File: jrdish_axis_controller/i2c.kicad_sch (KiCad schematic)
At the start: 18 parts, among them CN7 SM04B-SRSS-TB (LF)(SN), CN8 SM04B-SRSS-TB (LF)(SN), U5 LTC4311ISC6#TRPBF, U6 LM75BIMX-5/NOPB, U7 W25Q32JVSSIQ_C179173

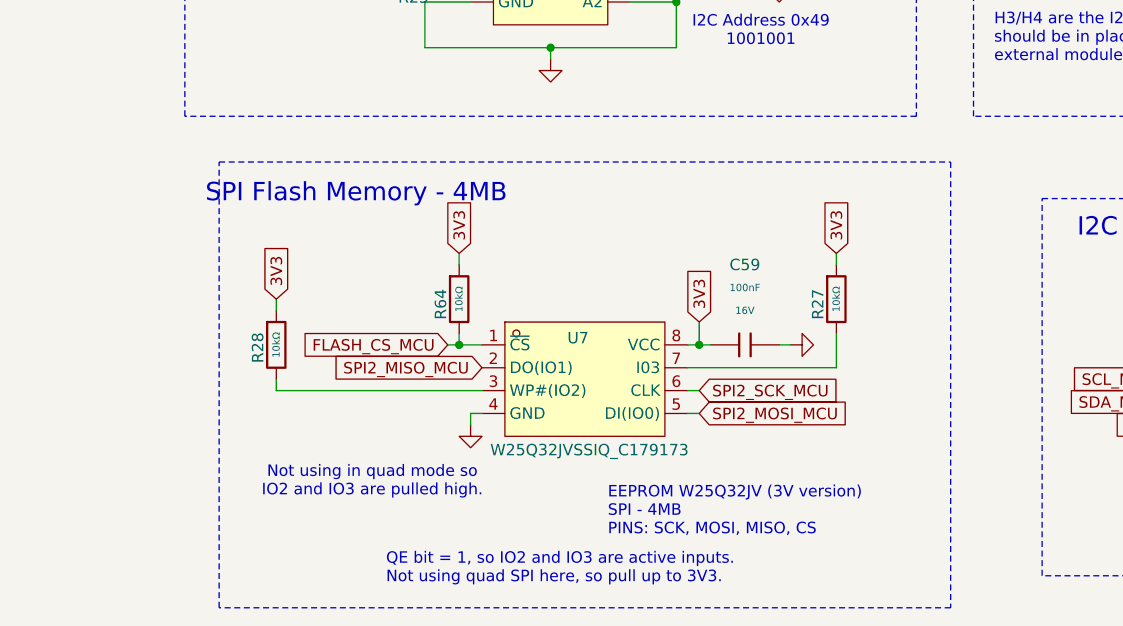
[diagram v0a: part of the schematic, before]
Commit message: Making refinements
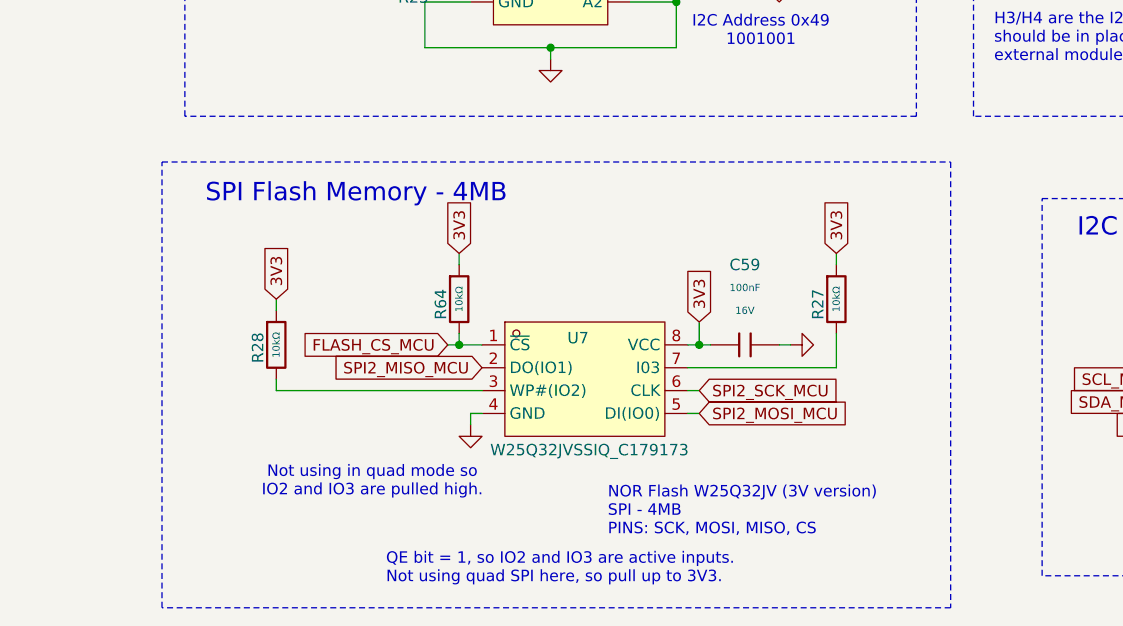
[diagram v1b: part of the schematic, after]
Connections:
- removed net GND: C55.2, C56.2, C57.2, C58.2, C59.2, CN7.1, CN7.5, CN7.6, CN8.1, CN8.5, CN8.6, U5.2 (GND), U5.5 (GND), U6.4 (GND), U6.5 (A2), U6.6 (A1), U7.4 (GND)
- new net: U6.4 (GND), U6.5 (A2), U6.6 (A1)
- new net: C55.2, C56.2, U5.2 (GND)
- new net: C57.2, C58.2
- new net: CN7.1, CN7.6, CN8.1, CN8.6
- new net: CN7.5, CN8.5
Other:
- note added: "NOR Flash W25Q32JV (3V version) SPI - 4MB PINS: SCK, MOSI, MISO, CS"
- note removed: "EEPROM W25Q32JV (3V version) SPI - 4MB PINS: SCK, MOSI, MISO, CS"
- title: (none) -> I2C and I2C Flash
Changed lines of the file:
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@@
 	(paper "A4")
 	(title_block
-		(date "2026-04-12")
+		(title "I2C and I2C Flash")
+		(date "2026-04-30")
 		(rev "1.0")
 		(company "JRSeti")
 	)
 	(rectangle
-		(start 66.04 100.33)
+		(start 59.69 100.33)
 		(end 147.32 149.86)
 		(stroke
@@
 		)
 	)
-	(text "EEPROM W25Q32JV (3V version) \nSPI - 4MB \nPINS: SCK, MOSI, MISO, CS"
+	(text "NOR Flash W25Q32JV (3V version) \nSPI - 4MB \nPINS: SCK, MOSI, MISO, CS"
 		(exclude_from_sim no)
 		(at 109.22 139.192 0)
@@
 			)
 		)
-		(property "Datasheet" "https://lcsc.com/product-detail/Others_JST-Sales-America__JST-Sales-America-SM04B-SRSS-TB-LF-SN_C160404.html"
+		(property "Datasheet" "https://www.lcsc.com/datasheet/C160404.pdf?spm=wm.sxq.inf.ggs&lcsc_vid=FFBaV1wHQFldUVICFgBfBVJTQVJWXgBfEQRYBAFQE1YxVlNRQFRYVVZVTllcVDtW"
 			(at 182.88 128.27 0)
 			(hide yes)
@@
 			)
 		)
-		(property "Datasheet" "https://lcsc.com/product-detail/Others_JST-Sales-America__JST-Sales-America-SM04B-SRSS-TB-LF-SN_C160404.html"
+		(property "Datasheet" "https://www.lcsc.com/datasheet/C160404.pdf?spm=wm.sxq.inf.ggs&lcsc_vid=FFBaV1wHQFldUVICFgBfBVJTQVJWXgBfEQRYBAFQE1YxVlNRQFRYVVZVTllcVDtW"
 			(at 212.09 128.27 0)
 			(hide yes)
